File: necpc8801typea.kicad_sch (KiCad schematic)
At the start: 263 parts, among them J4 Conn_01x04, Q1 Q_PMOS_GSD AO3401A, Q2 Q_NMOS_GSD 2N7002, Q3 Q_NMOS_GSD 2N7002, SW1 SW_Push, U1 AMS1117-3.3, U2 TPS2553DBVR, U3 STM32F401RETx, U4 24LC64, U5 USBLC6-2SC6, Y1 16MHz

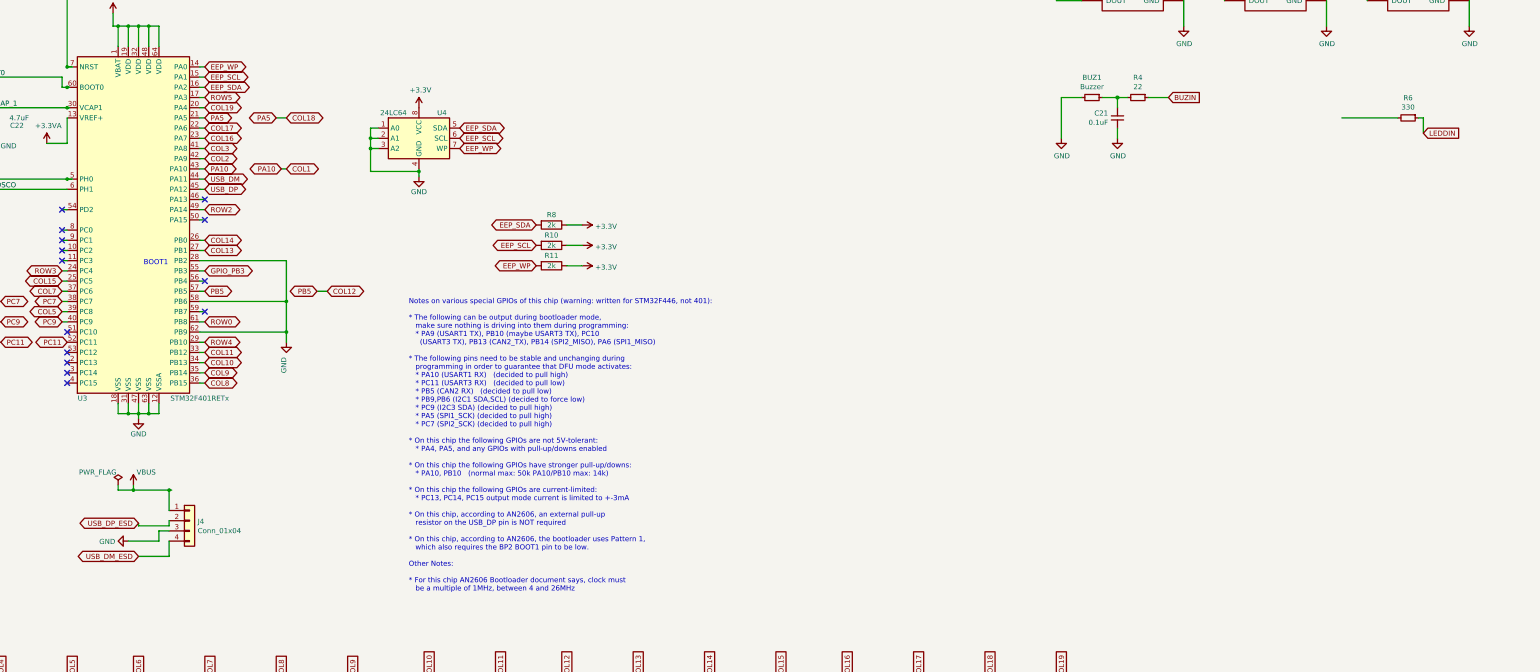
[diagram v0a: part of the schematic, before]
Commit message: updates
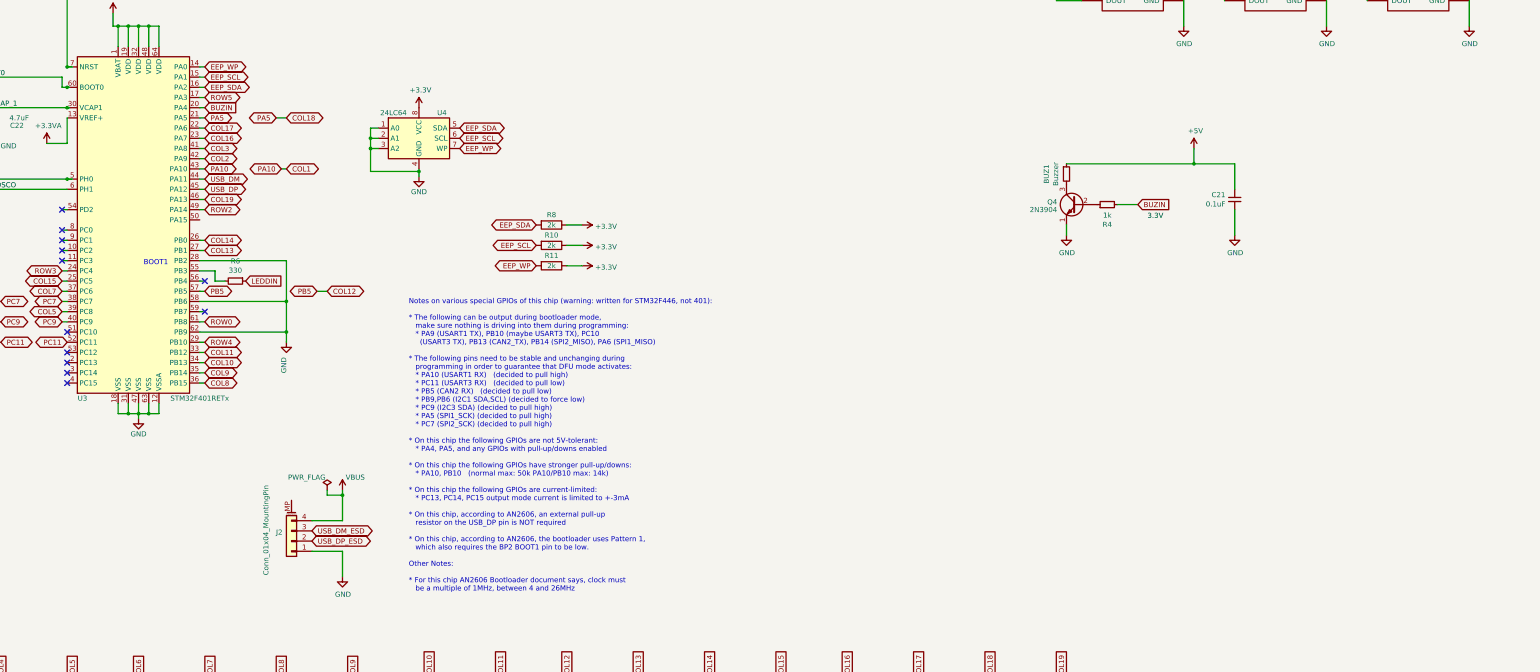
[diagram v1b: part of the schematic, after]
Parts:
- removed J4: Conn_01x04, Connector_JST:JST_PH_S4B-PH-K_1x04_P2.00mm_Horizontal, symbol controller-rescue:Conn_01x04-Connector_Generic
- added J2: Conn_01x04_MountingPin, Connector_JST:JST_SH_SM04B-SRSS-TB_1x04-1MP_P1.00mm_Horizontal, symbol Connector_Generic_MountingPin:Conn_01x04_MountingPin
- added Q4: 2N3904, Package_TO_SOT_SMD:SOT-23, symbol Transistor_BJT:2N3904
- R4: value 22 -> 1k
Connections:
- net GPIO_PB3 is gone; now on an unnamed net: U3.55 (PB3)
- net +5V: now also BUZ1.1, C21.1
- net BUZIN: now also R4.2, U3.20 (PA4); no longer R4.1
- net COL19: now also U3.46 (PA13); no longer U3.20 (PA4)
- net GND: now also J2.1 (Pin_1), Q4.1 (E); no longer BUZ1.2
- net USB_DM_ESD: now also J2.3 (Pin_3)
- net USB_DP_ESD: now also J2.2 (Pin_2)
- net VBUS: now also J2.4 (Pin_4)
- new net: BUZ1.2, Q4.3 (C)
- new net: Q4.2 (B), R4.1
- no-connect marks 16 -> 14
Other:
- moved on the sheet: BUZ1, C21, R4, R6
